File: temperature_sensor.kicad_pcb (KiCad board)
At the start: 2 copper layers, 18 parts, among them SW1 500SSP3S1M2QEA, U3 XIAO-SAMD21-SMD, U5 TMP37FT9Z

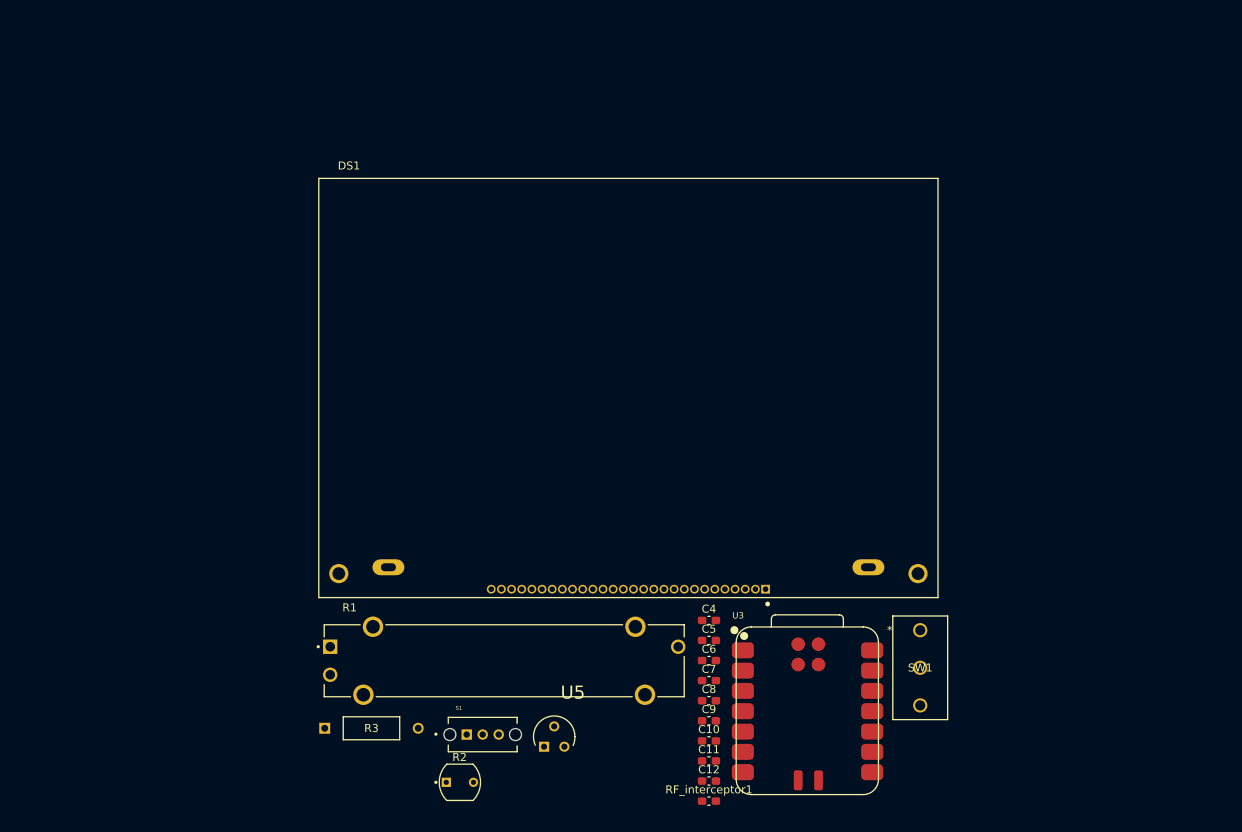
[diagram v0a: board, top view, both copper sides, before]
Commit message: initial pcb design
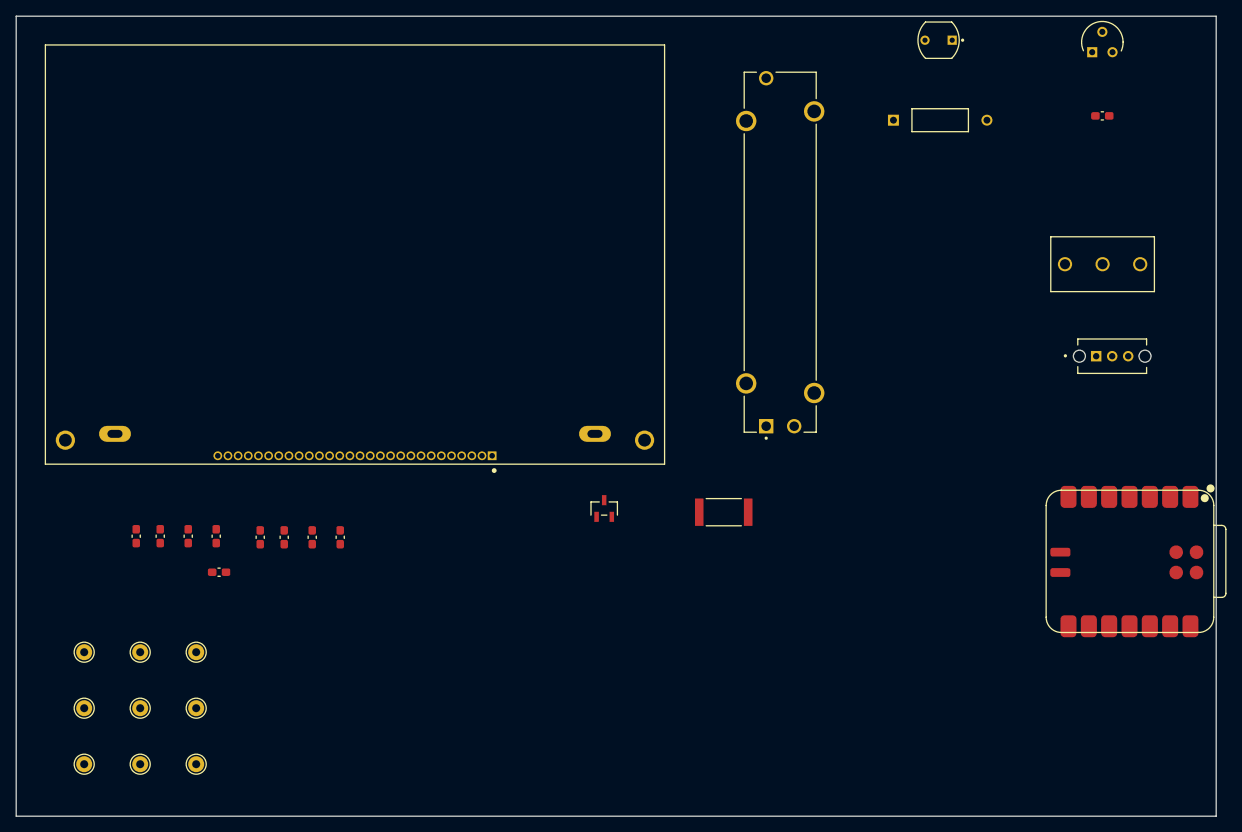
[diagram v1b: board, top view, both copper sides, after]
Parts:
- added R4: 820, 1_my_custom_library:RESC6332X65N, F.Cu at (128.9, 87.5)
- added TP1: gnd_TP, Connector_Pin:Pin_D1.0mm_L10.0mm, F.Cu at (49.0, 112.0)
- added TP2: pot_TP, Connector_Pin:Pin_D1.0mm_L10.0mm, F.Cu at (63.0, 119.0)
- added TP3: photoresistor_TP, Connector_Pin:Pin_D1.0mm_L10.0mm, F.Cu at (63.0, 105.0)
- added TP4: PWM_TP, Connector_Pin:Pin_D1.0mm_L10.0mm, F.Cu at (56.0, 112.0)
- added TP5: K_TP, Connector_Pin:Pin_D1.0mm_L10.0mm, F.Cu at (63.0, 112.0)
- added TP6: SCL_TP, Connector_Pin:Pin_D1.0mm_L10.0mm, F.Cu at (56.0, 119.0)
- added TP7: SI_TP, Connector_Pin:Pin_D1.0mm_L10.0mm, F.Cu at (49.0, 119.0)
- added TP8: fahrenheit_celsius_TP, Connector_Pin:Pin_D1.0mm_L10.0mm, F.Cu at (56.0, 105.0)
- added TP9: 3v3_TP, Connector_Pin:Pin_D1.0mm_L10.0mm, F.Cu at (49.0, 105.0)
- added U1: MMBT3904LT1G, 1_my_custom_library:SOT-23_3L_ONS, F.Cu at (114.0, 87.0)
- moved U5 110.6 mm to (177.5, 27.5)
- moved R2 110.4 mm to (155.8, 28.5), turned to 180 degrees
- moved R3 104.1 mm to (150.2, 38.5)
- moved RF_interceptor1 98.8 mm to (176.3, 38.0), turned to 180 degrees
- moved S1 91.8 mm to (177.5, 68.0)
- moved C6 73.3 mm to (55.5, 90.5), turned to 90 degrees
- moved C5 69.8 mm to (58.5, 90.5), turned to 90 degrees
- moved C4 65.9 mm to (62.0, 90.5), turned to 90 degrees
- moved C8 64.9 mm to (65.5, 90.5), turned to 90 degrees
- moved C7 62.7 mm to (65.9, 95.0)
- moved R1 61.6 mm to (136.0, 55.0), turned to 90 degrees
- moved C10 61.6 mm to (71.0, 90.6), turned to 90 degrees
- moved C12 61.2 mm to (74.0, 90.6), turned to 90 degrees
- moved C11 56.9 mm to (77.5, 90.6), turned to 90 degrees
- moved U3 54.3 mm to (169.2, 84.8), turned to -90 degrees
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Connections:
- DS1 pad A: Net-(U3-PA02_A0_D0) -> Net-(DS1-C86)
- DS1 pad K: GND -> Net-(U1-COLLECTOR)
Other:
- board outline added: 150 x 100 mm
